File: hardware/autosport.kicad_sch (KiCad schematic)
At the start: 11 parts

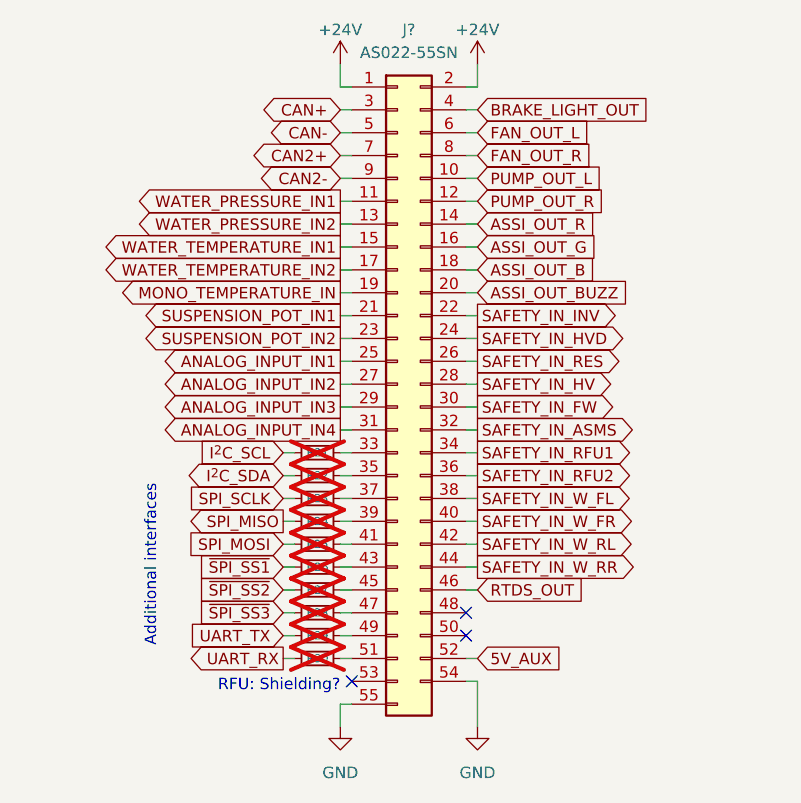
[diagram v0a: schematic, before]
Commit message: Add the Cube project
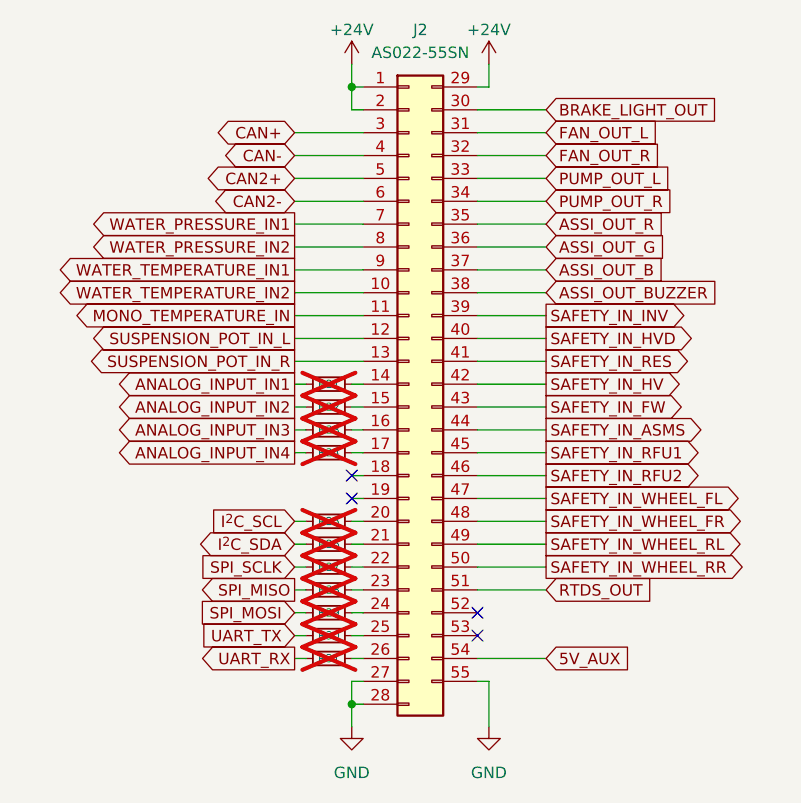
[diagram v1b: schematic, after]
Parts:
- removed J?: AS022-55SN, symbol Connector_Generic:Conn_2Rows-55Pins
- removed R26, R27, R28: 0R, symbol Device:R_Small
- added J2: AS022-55SN, Local_Library:AS022-55SN, symbol AS022-55SN:AS022-55SN
- added R21, R22, R23, R24: 0R, symbol Device:R_Small
- renumbered R21 to R25, R22 to R26, R23 to R27, R24 to R28, R25 to R29, R29 to R30, R30 to R31
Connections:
- net +24V: now also J2.1 (Pin_1), J2.2 (Pin_2), J2.29 (Pin_29)
- net 5V_AUX: now also J2.54 (Pin_54)
- net ANALOG_INPUT_IN1: now also R21.1
- net ANALOG_INPUT_IN2: now also R22.1
- net ANALOG_INPUT_IN3: now also R23.1
- net ANALOG_INPUT_IN4: now also R24.1
- net ASSI_OUT_B: now also J2.37 (Pin_37)
- net ASSI_OUT_G: now also J2.36 (Pin_36)
- net ASSI_OUT_R: now also J2.35 (Pin_35)
- net BRAKE_LIGHT_OUT: now also J2.30 (Pin_30)
- net CAN+: now also J2.3 (Pin_3)
- net CAN-: now also J2.4 (Pin_4)
- net CAN2+: now also J2.5 (Pin_5)
- net CAN2-: now also J2.6 (Pin_6)
- net FAN_OUT_L: now also J2.31 (Pin_31)
- net FAN_OUT_R: now also J2.32 (Pin_32)
- net GND: now also J2.27 (Pin_27), J2.28 (Pin_28), J2.55 (Pin_55)
- net MONO_TEMPERATURE_IN: now also J2.11 (Pin_11)
- net PUMP_OUT_L: now also J2.33 (Pin_33)
- net PUMP_OUT_R: now also J2.34 (Pin_34)
- net RTDS_OUT: now also J2.51 (Pin_51)
- net SAFETY_IN_ASMS: now also J2.44 (Pin_44)
- net SAFETY_IN_FW: now also J2.43 (Pin_43)
- net SAFETY_IN_HV: now also J2.42 (Pin_42)
- net SAFETY_IN_HVD: now also J2.40 (Pin_40)
- net SAFETY_IN_INV: now also J2.39 (Pin_39)
- net SAFETY_IN_RES: now also J2.41 (Pin_41)
- net SAFETY_IN_RFU1: now also J2.45 (Pin_45)
- net SAFETY_IN_RFU2: now also J2.46 (Pin_46)
- net WATER_PRESSURE_IN1: now also J2.7 (Pin_7)
- net WATER_PRESSURE_IN2: now also J2.8 (Pin_8)
- net WATER_TEMPERATURE_IN1: now also J2.9 (Pin_9)
- net WATER_TEMPERATURE_IN2: now also J2.10 (Pin_10)
- net at R26.2: now also J2.21 (Pin_21)
- net at R29.2: now also J2.24 (Pin_24)
- net at R27.2: now also J2.22 (Pin_22)
- net at R25.2: now also J2.20 (Pin_20)
- net at R28.2: now also J2.23 (Pin_23)
- net at R30.2: now also J2.25 (Pin_25)
- net at R31.2: now also J2.26 (Pin_26)
- new net: J2.14 (Pin_14), R21.2
- new net: J2.15 (Pin_15), R22.2
- new net: J2.16 (Pin_16), R23.2
- new net: J2.17 (Pin_17), R24.2
- new net ASSI_OUT_BUZZER: J2.38 (Pin_38)
- new net SAFETY_IN_WHEEL_FL: J2.47 (Pin_47)
- new net SAFETY_IN_WHEEL_FR: J2.48 (Pin_48)
- new net SAFETY_IN_WHEEL_RL: J2.49 (Pin_49)
- new net SAFETY_IN_WHEEL_RR: J2.50 (Pin_50)
- new net SUSPENSION_POT_IN_L: J2.12 (Pin_12)
- new net SUSPENSION_POT_IN_R: J2.13 (Pin_13)
- no-connect marks 3 -> 4
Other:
- note removed: "Additional interfaces"
- note removed: "RFU: Shielding?"
- moved on the sheet: R25, R26, R27, R28, R29, R30, R31
